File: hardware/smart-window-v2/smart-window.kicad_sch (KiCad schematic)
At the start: 57 parts, among them J1 Screw_Terminal_01x02, J10 Conn_01x06_Pin, J11 Conn_02x03_Odd_Even, J12 Conn_01x04_Socket, J13 Conn_01x04_Socket, J14 Conn_01x05_Pin, J15 Conn_01x03_Socket, J2 12V INPUT, J3 Screw_Terminal_01x02, J4 Conn_01x03_Socket, J5 Conn_01x03_Socket, J6 Screw_Terminal_01x02, J7 Conn_01x04_Socket, J8 Conn_01x04_Socket, J9 Conn_01x04_Socket, SW1 SW_Push_Dual, SW2 SW_Push_Dual, U1 TSDP341xx, U2 DHT11, U3 L7805, U4 ATmega328P-P, Y1 16MHz

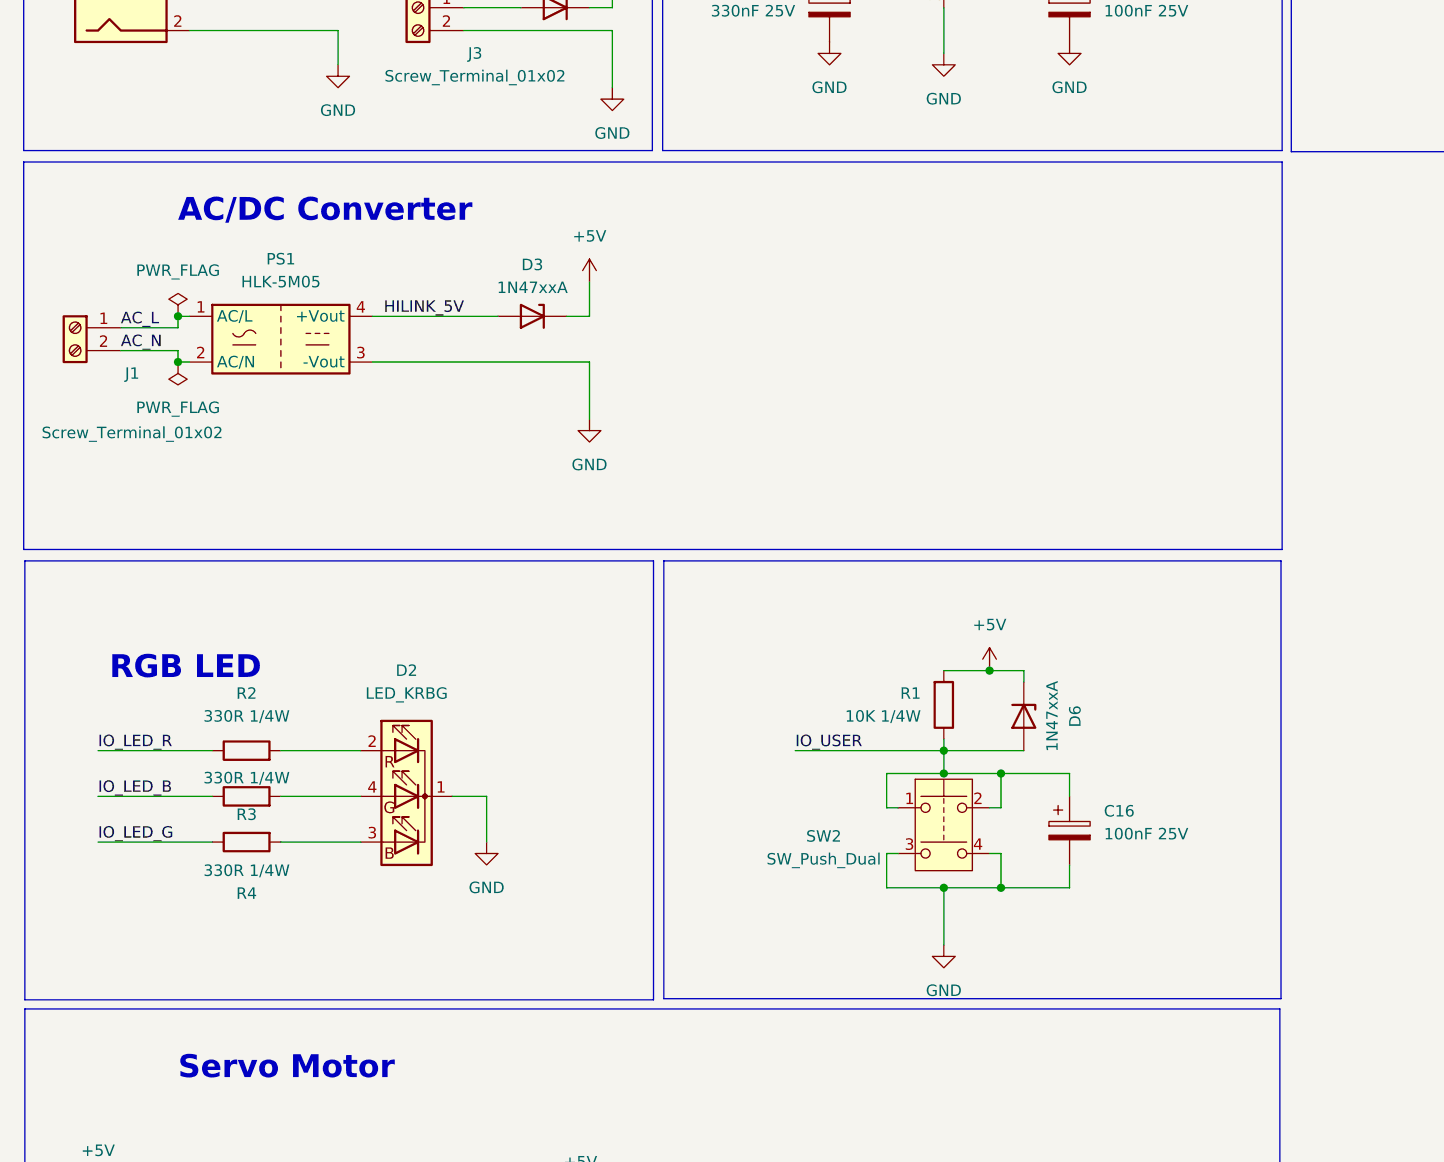
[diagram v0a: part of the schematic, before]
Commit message: Schematic Completed
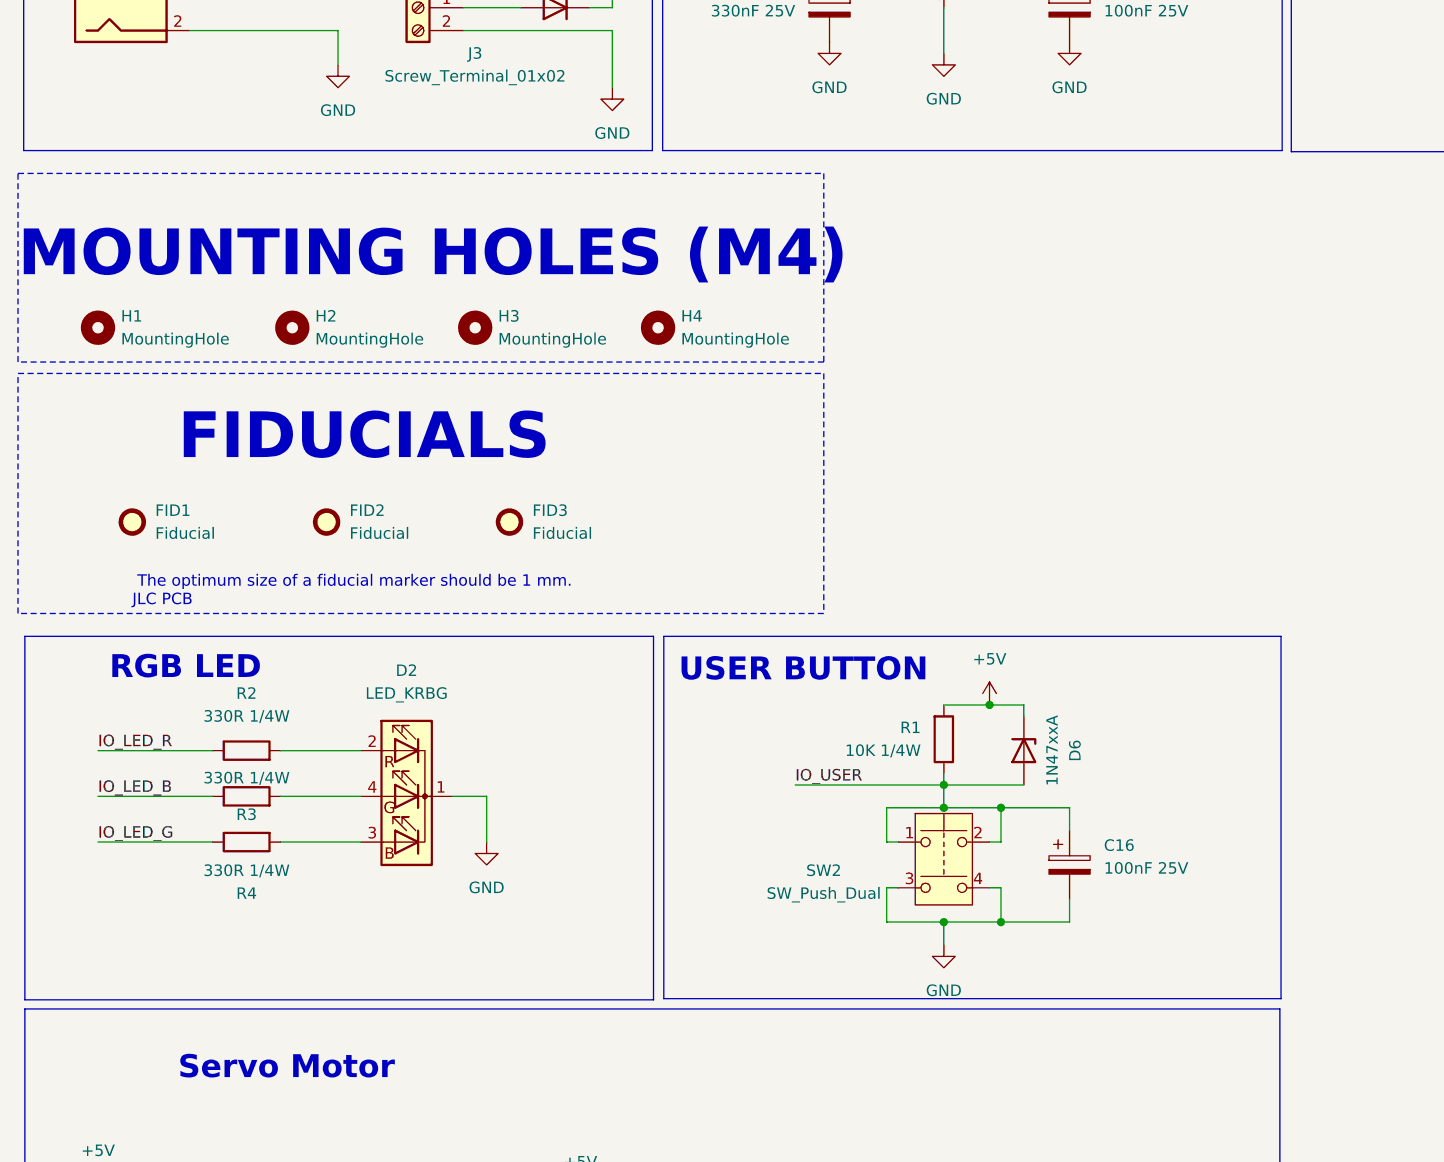
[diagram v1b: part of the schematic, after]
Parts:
- removed D3: 1N47xxA, Diode_THT:D_DO-41_SOD81_P10.16mm_Horizontal, symbol Diode:1N47xxA
- removed J1: Screw_Terminal_01x02, TerminalBlock:TerminalBlock_bornier-2_P5.08mm, symbol Connector:Screw_Terminal_01x02
- removed PS1: HLK-5M05, Converter_ACDC:Converter_ACDC_Hi-Link_HLK-5Mxx, symbol Converter_ACDC:HLK-5M05
- added FID1, FID2, FID3: Fiducial, Fiducial:Fiducial_1mm_Mask2mm, symbol Mechanical:Fiducial
- added H1, H2, H3, H4: MountingHole, MountingHole:MountingHole_4.3mm_M4, symbol Mechanical:MountingHole
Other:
- note added: "FIDUCIALS"
- note added: "MOUNTING HOLES (M4)"
- note added: "The optimum size of a fiducial marker should be 1 mm. JLC PCB"
- note added: "USER BUTTON"
- note removed: "AC/DC Converter"
- moved on the sheet: C16, D6, R1, SW2
